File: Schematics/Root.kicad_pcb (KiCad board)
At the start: 2 copper layers, 100 x 100 mm, 133 parts, among them CON1 USB-MICRO-B, CON2 BARREL_JACK, IC1 ATXMEGA256A3BU-A, J1 AVR_JTAG_Header, P1 CONN_02X08, U1 PCA9685, U10 PCA9685, U11 PCA9685, U12 PCA9685, U13 LT8612, U2 PCA9685, U3 PCA9685, U4 PCA9685, U5 PCA9685, U6 PCA9685, U7 PCA9685, U8 PCA9685, U9 PCA9685, X1 16MHz, X2 32.768KhZ

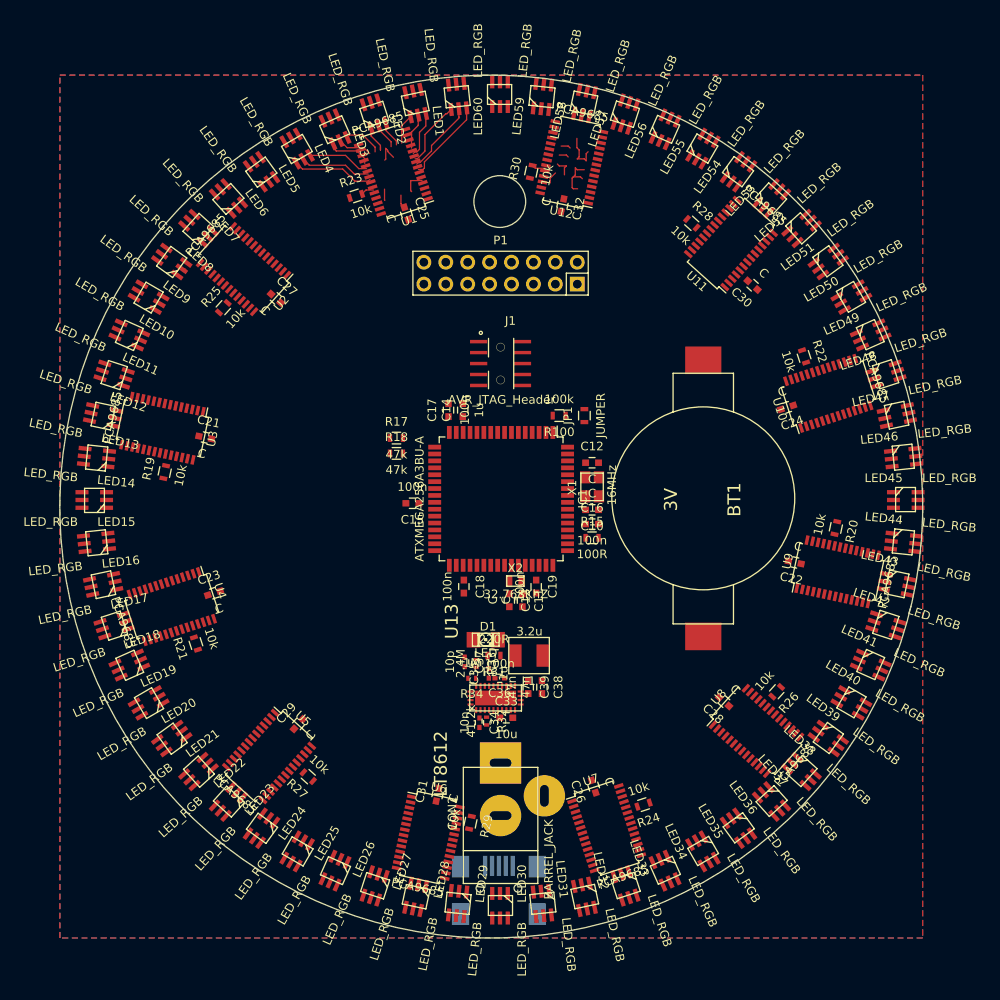
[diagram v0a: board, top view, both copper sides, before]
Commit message: Ammended a net. Done a lot of routing
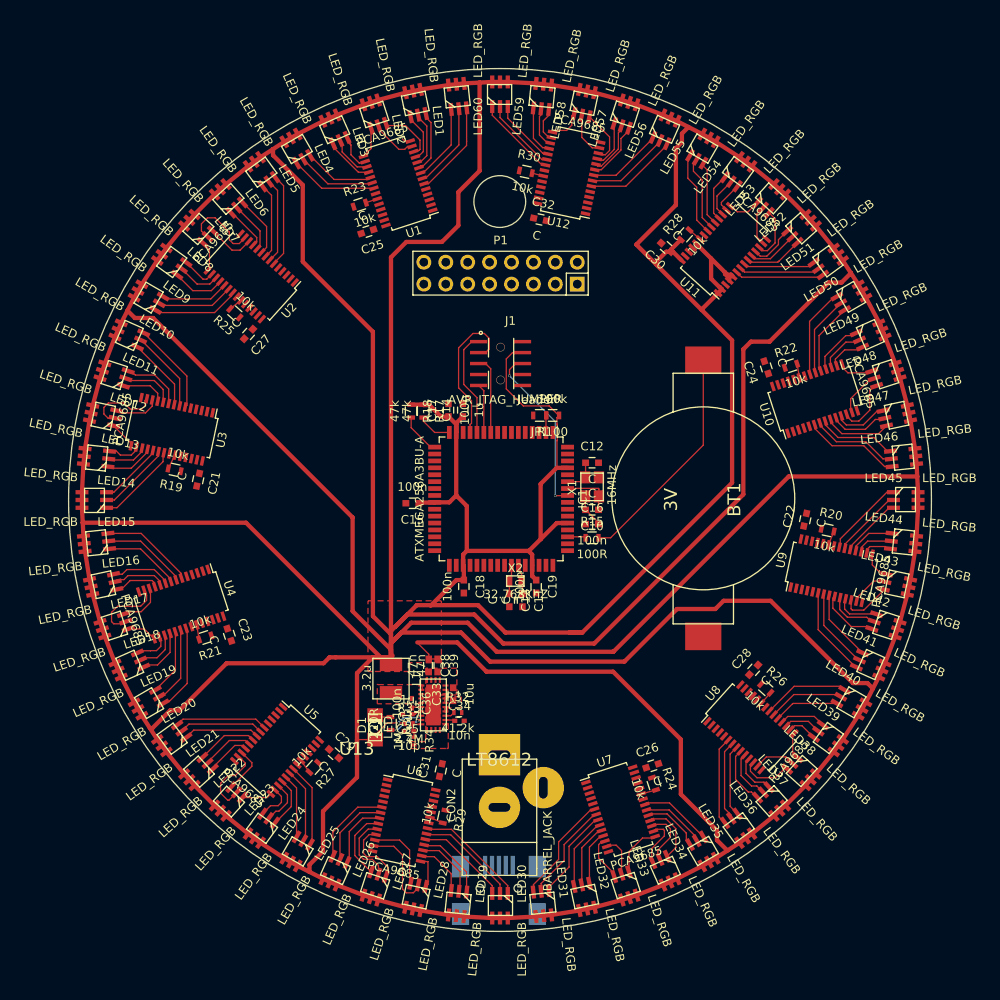
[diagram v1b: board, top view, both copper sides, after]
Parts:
- moved D1 16.4 mm to (91.0, 111.6), turned to 90 degrees
- moved L1 16.2 mm to (92.9, 105.9), turned to 90 degrees
- moved R31 14.4 mm to (92.8, 111.1), turned to 270 degrees
- moved C38 13.4 mm to (97.2, 104.4)
- moved C30 10.9 mm to (124.7, 55.9)
- moved C39 10.8 mm to (98.3, 104.4)
- moved C36 10.6 mm to (95.3, 108.8), turned to 270 degrees
- moved C35 10.5 mm to (94.8, 110.0), turned to 180 degrees
- moved R33 10.4 mm to (95.0, 111.1), turned to 0 degrees
- moved C37 10.3 mm to (95.0, 112.0), turned to 0 degrees
- moved R34 9.89 mm to (95.5, 113.1), turned to 270 degrees
- moved U13 7.25 mm to (97.8, 109.0), turned to 180 degrees
- moved C26 7.21 mm to (123.2, 116.0), turned to 18 degrees
- moved C33 6.74 mm to (100.1, 107.7), turned to 90 degrees
- moved C29 5.37 mm to (86.3, 114.6), turned to 318 degrees
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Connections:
- IC1 pad 2: Net-(IC1-Pad2) -> /Microcontroller/JUMPER
- JP1 pad 1: Net-(JP1-Pad1) -> /Microcontroller/JUMPER
- R100 pad 2: Net-(JP1-Pad1) -> /Microcontroller/JUMPER
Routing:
- net VPP: track 1.57 -> 1092.9 mm, vias 0 -> 2
- net Net-(BT1-Pad1): track 0.00 -> 26.4 mm
- net (no net): track 23.0 -> 0.00 mm
- net /Microcontroller/~RESET: track 0.00 -> 20.0 mm, vias 0 -> 2
- net /Microcontroller/TDO: track 0.00 -> 17.6 mm
- net Net-(LED30-PadBC): track 0.00 -> 12.9 mm
- net Net-(LED31-PadRC): track 0.00 -> 12.8 mm
- net /Microcontroller/TCK: track 0.00 -> 12.3 mm
- net Net-(LED30-PadGC): track 0.00 -> 12.0 mm
- net Net-(LED31-PadGC): track 0.00 -> 11.7 mm
- net Net-(LED46-PadRC): track 0.00 -> 11.2 mm
- net Net-(LED16-PadRC): track 0.00 -> 11.0 mm
- net Net-(LED6-PadRC): track 0.00 -> 10.9 mm
- net Net-(LED56-PadRC): track 0.00 -> 10.9 mm
- net Net-(LED30-PadRC): track 0.00 -> 10.9 mm
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- added copper zone on F.Cu, net /Power Supply/SW
- added copper zone on F.Cu, net /Power Supply/Vin
- added copper zone on F.Cu, net VPP
- removed copper zone on B.Cu, net GND
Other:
- outline, holes or cut-outs redrawn
- net class Power added: clearance 0.15, trace_width 0.5, via_dia 0.3, via_drill 0.25
